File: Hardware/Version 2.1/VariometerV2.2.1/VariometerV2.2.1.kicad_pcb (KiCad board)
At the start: 4 copper layers, 95.9 x 70.5 mm, 157 parts, among them IC1 ESP32-S3-WROOM, IC3 BQ24196RGER, IC4 TPS22916CNYFPR, IC5 TPS73701DCQR, J1 USB_C_Receptacle_USB2.0, J2 Conn_01x02, J4 FFC24/0.5MM, J5 U.FL-R-SMT(01), J6 SW, J7 Conn_01x02, J8 LED_CHRG, J9 SW, Q1 AO3401A, Q2 AO3401A, Q3 AO3400A, Q4 AO3400A, SW3 BTN1, SW4 BTN1, SW5 BTN1, SW6 BTN1, U1 SRV05-4, U2 SRV05-4, U3 SRV05-4, U4 DPS310, U5 BMI088, U6 QMC5883L, U7 MAX98357A, U8 L76-L

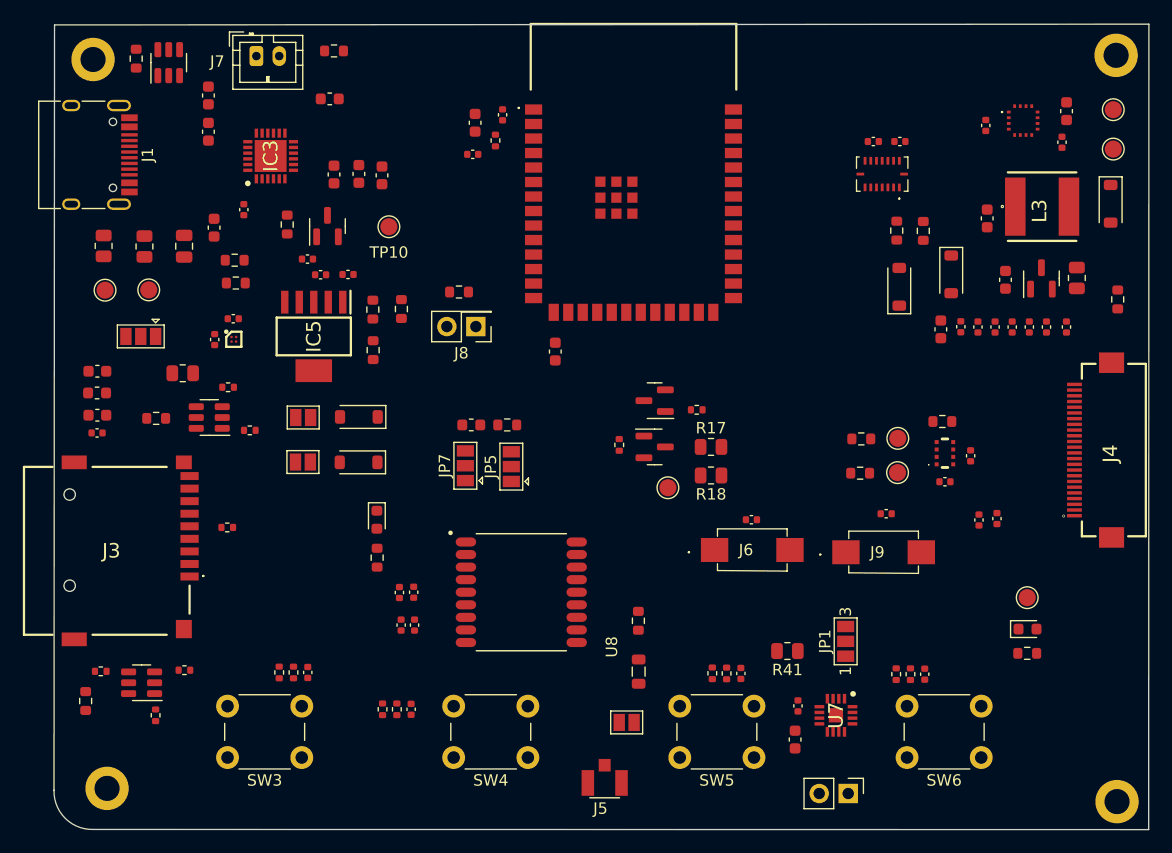
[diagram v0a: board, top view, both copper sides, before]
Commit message: WRL File
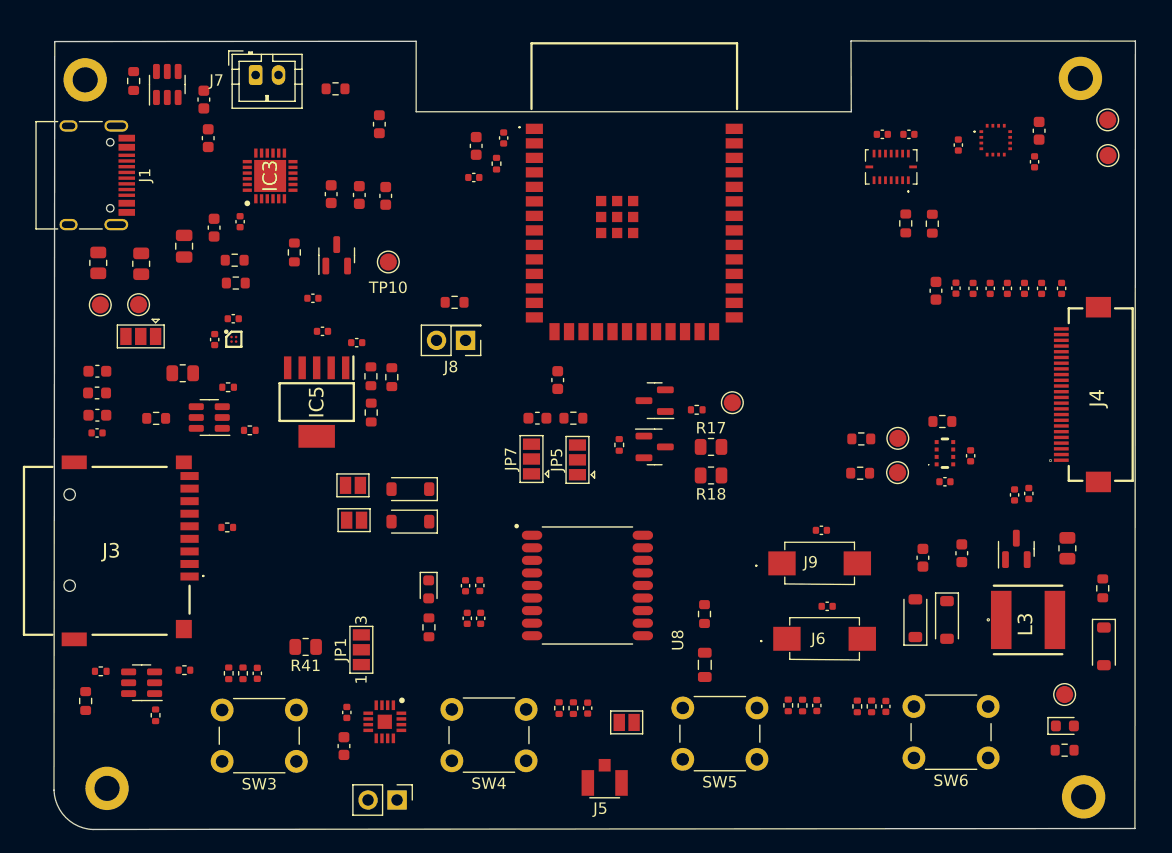
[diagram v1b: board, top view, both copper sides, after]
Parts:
- moved JP1 42.4 mm to (131.3, 105.9)
- moved R41 42.2 mm to (126.4, 105.7)
- moved C42 39.5 mm to (129.7, 114.3)
- moved C43 39.5 mm to (130.0, 111.4)
- moved J2 39.5 mm to (134.4, 119.1)
- moved U7 39.5 mm to (133.3, 112.2)
- moved D3 38.8 mm to (196.3, 105.6)
- moved L3 36.2 mm to (189.6, 103.3)
- moved D4 30.3 mm to (182.5, 103.3)
- moved C33 30.2 mm to (180.4, 97.9)
- moved D5 29.1 mm to (179.8, 103.1)
- moved R35 25.3 mm to (196.2, 100.5)
- moved C34 24.2 mm to (183.8, 97.5)
- moved Q4 23.8 mm to (188.6, 97.1)
- moved R34 23.7 mm to (193.1, 97.0)
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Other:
- board size 95.9 x 70.5 mm -> 94.7 x 69.1 mm
